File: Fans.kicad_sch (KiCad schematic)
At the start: 12 parts, among them Q1 NMOS, Q2 NMOS

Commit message: Initial layout with 1 pump, 2 temp, 1 flow all on front side
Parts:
- Q1, Q2: footprint Package_TO_SOT_SMD:LFPAK33 -> Package_TO_SOT_SMD:SOT-23
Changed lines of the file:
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@@
+	)
+	(symbol
+		(lib_id "power:GND")
+		(at 114.3 63.5 0)
+		(unit 1)
+		(exclude_from_sim no)
+		(in_bom yes)
+		(on_board yes)
+		(dnp no)
+		(fields_autoplaced yes)
+		(property "Reference" "#PWR016"
+			(at 114.3 69.85 0)
+			(effects
+				(font
+					(size 1.27 1.27)
+				)
+				(hide yes)
+			)
+		)
+		(property "Value" "GND"
+			(at 114.3 68.58 0)
+			(effects
+				(font
+					(size 1.27 1.27)
+				)
+			)
+		)
+		(property "Footprint" ""
+			(at 114.3 63.5 0)
+			(effects
+				(font
+					(size 1.27 1.27)
+				)
+				(hide yes)
+			)
+		)
+		(property "Datasheet" ""
+			(at 114.3 63.5 0)
+			(effects
+				(font
+					(size 1.27 1.27)
+				)
+				(hide yes)
+			)
+		)
+		(property "Description" "Power symbol creates a global label with name \"GND\" , ground"
+			(at 114.3 63.5 0)
+			(effects
+				(font
+					(size 1.27 1.27)
+				)
+				(hide yes)
+			)
+		)
+		(pin "1"
+		)
+		(instances
+			(project "PTN-PumpControlBoard"
+				(path "/591f46f8-eb1d-42dc-a4cb-8182eac4ef58/d90f7da4-ca39-48c6-8d97-b8d1e37c7dd0"
+					(reference "#PWR016")
+					(unit 1)
+				)
+			)
+		)
+	)
+	(symbol
+		(lib_id "Device:R_US")
+		(at 113.03 114.3 0)
+		(unit 1)
+		(exclude_from_sim no)
+		(in_bom yes)
+		(on_board yes)
+		(dnp no)
+		(property "Reference" "R8"
+			(at 115.57 113.0299 0)
+			(effects
+				(font
+					(size 1.27 1.27)
+				)
+				(justify left)
+			)
+		)
+		(property "Value" "1k"
+			(at 115.57 115.5699 0)
+			(effects
+				(font
+					(size 1.27 1.27)
+				)
+				(justify left)
+			)
+		)
+		(property "Footprint" "Resistor_SMD:R_0805_2012Metric"
+			(at 114.046 114.554 90)
+			(effects
+				(font
+					(size 1.27 1.27)
+				)
+				(hide yes)
+			)
+		)
+		(property "Datasheet" "~"
+			(at 113.03 114.3 0)
+			(effects
+				(font
+					(size 1.27 1.27)
+				)
+				(hide yes)
+			)
+		)
+		(property "Description" "Resistor, US symbol"
+			(at 113.03 114.3 0)
+			(effects
+				(font
+					(size 1.27 1.27)
+				)
+				(hide yes)
+			)
+		)
+		(pin "1"
+		)
+		(pin "2"
+		)
+		(instances
+			(project "PTN-PumpControlBoard"
+				(path "/591f46f8-eb1d-42dc-a4cb-8182eac4ef58/d90f7da4-ca39-48c6-8d97-b8d1e37c7dd0"
+					(reference "R8")
+					(unit 1)
+				)
+			)
+		)
+	)
+	(symbol
+		(lib_id "Device:D")
+		(at 52.07 38.1 270)
+		(unit 1)
+		(exclude_from_sim no)
+		(in_bom yes)
+		(on_board yes)
+		(dnp no)
+		(fields_autoplaced yes)
+		(property "Reference" "D1"
+			(at 54.61 36.8299 90)
+			(effects
+				(font
+					(size 1.27 1.27)
+				)
+				(justify left)
+			)
+		)
+		(property "Value" "1N4448W"
+			(at 54.61 39.3699 90)
+			(effects
+				(font
+					(size 1.27 1.27)
+				)
+				(justify left)
+			)
+		)
+		(property "Footprint" "Diode_SMD:D_SOD-323"
+			(at 52.07 38.1 0)
+			(effects
+				(font
+					(size 1.27 1.27)
+				)
+				(hide yes)
+			)
+		)
+		(property "Datasheet" "https://www.vishay.com/docs/85722/1n4448w.pdf"
+			(at 52.07 38.1 0)
+			(effects
+				(font
+					(size 1.27 1.27)
+				)
+				(hide yes)
+			)
+		)
+		(property "Description" "Diode"
+			(at 52.07 38.1 0)
+			(effects
+				(font
+					(size 1.27 1.27)
+				)
+				(hide yes)
+			)
+		)
+		(property "Sim.Device" "D"
+			(at 52.07 38.1 0)
+			(effects
+				(font
+					(size 1.27 1.27)
+				)
+				(hide yes)
+			)
+		)
+		(property "Sim.Pins" "1=K 2=A"
+			(at 52.07 38.1 0)
+			(effects
+				(font
+					(size 1.27 1.27)
+				)
+				(hide yes)
+			)
+		)
+		(pin "1"
+		)
+		(pin "2"
+		)
+		(instances
+			(project "PTN-PumpControlBoard"
+				(path "/591f46f8-eb1d-42dc-a4cb-8182eac4ef58/d90f7da4-ca39-48c6-8d97-b8d1e37c7dd0"
+					(reference "D1")
+					(unit 1)
+				)
+			)
+		)
 	)
 	(symbol
@@
 			)
 		)
-		(property "Footprint" "Package_TO_SOT_SMD:LFPAK33"
+		(property "Footprint" "Package_TO_SOT_SMD:SOT-23"
 			(at 66.04 50.8 0)
 			(effects
@@
 	)
 	(symbol
-		(lib_id "power:GND")
-		(at 114.3 63.5 0)
-		(unit 1)
-		(exclude_from_sim no)
-		(in_bom yes)
-		(on_board yes)
-		(dnp no)
-		(fields_autoplaced yes)
-		(property "Reference" "#PWR016"
-			(at 114.3 69.85 0)
-			(effects
-				(font
-					(size 1.27 1.27)
-				)
-				(hide yes)
-			)
-		)
-		(property "Value" "GND"
-			(at 114.3 68.58 0)
-			(effects
-				(font
-					(size 1.27 1.27)
-				)
-			)
-		)
-		(property "Footprint" ""
-			(at 114.3 63.5 0)
-			(effects
-				(font
-					(size 1.27 1.27)
-				)
-				(hide yes)
-			)
-		)
-		(property "Datasheet" ""
-			(at 114.3 63.5 0)
-			(effects
-				(font
-					(size 1.27 1.27)
-				)
-				(hide yes)
-			)
-		)
-		(property "Description" "Power symbol creates a global label with name \"GND\" , ground"
-			(at 114.3 63.5 0)
-			(effects
-				(font
-					(size 1.27 1.27)
-				)
-				(hide yes)
-			)
-		)
-		(pin "1"
-		)
-		(instances
-			(project "PTN-PumpControlBoard"
-				(path "/591f46f8-eb1d-42dc-a4cb-8182eac4ef58/d90f7da4-ca39-48c6-8d97-b8d1e37c7dd0"
-					(reference "#PWR016")
-					(unit 1)
-				)
-			)
-		)
-	)
-	(symbol
-		(lib_id "Device:R_US")
-		(at 113.03 114.3 0)
-		(unit 1)
-		(exclude_from_sim no)
-		(in_bom yes)
-		(on_board yes)
-		(dnp no)
-		(property "Reference" "R8"
-			(at 115.57 113.0299 0)
-			(effects
-				(font
-					(size 1.27 1.27)
-				)
-				(justify left)
-			)
-		)
-		(property "Value" "1k"
-			(at 115.57 115.5699 0)
-			(effects
-				(font
-					(size 1.27 1.27)
-				)
-				(justify left)
-			)
-		)
-		(property "Footprint" "Resistor_SMD:R_0805_2012Metric"
-			(at 114.046 114.554 90)
-			(effects
-				(font
-					(size 1.27 1.27)
-				)
-				(hide yes)
-			)
-		)
-		(property "Datasheet" "~"
-			(at 113.03 114.3 0)
-			(effects
-				(font
-					(size 1.27 1.27)
-				)
-				(hide yes)
-			)
-		)
-		(property "Description" "Resistor, US symbol"
-			(at 113.03 114.3 0)
-			(effects
-				(font
-					(size 1.27 1.27)
-				)
-				(hide yes)
-			)
-		)
-		(pin "1"
-		)
-		(pin "2"
-		)
-		(instances
-			(project "PTN-PumpControlBoard"
-				(path "/591f46f8-eb1d-42dc-a4cb-8182eac4ef58/d90f7da4-ca39-48c6-8d97-b8d1e37c7dd0"
-					(reference "R8")
-					(unit 1)
-				)
-			)
-		)
-	)
-	(symbol
-		(lib_id "Device:D")
-		(at 52.07 38.1 270)
-		(unit 1)
-		(exclude_from_sim no)
-		(in_bom yes)
-		(on_board yes)
-		(dnp no)
-		(fields_autoplaced yes)
-		(property "Reference" "D1"
-			(at 54.61 36.8299 90)
-			(effects
-				(font
-					(size 1.27 1.27)
-				)
-				(justify left)
-			)
-		)
-		(property "Value" "1N4448W"
-			(at 54.61 39.3699 90)
-			(effects
-				(font
-					(size 1.27 1.27)
-				)
-				(justify left)
-			)
-		)
-		(property "Footprint" "Diode_SMD:D_SOD-323"
-			(at 52.07 38.1 0)
-			(effects
-				(font
-					(size 1.27 1.27)
-				)
-				(hide yes)
-			)
-		)
-		(property "Datasheet" "https://www.vishay.com/docs/85722/1n4448w.pdf"
-			(at 52.07 38.1 0)
-			(effects
-				(font
-					(size 1.27 1.27)
-				)
-				(hide yes)
-			)
-		)
-		(property "Description" "Diode"
-			(at 52.07 38.1 0)
-			(effects
-				(font
-					(size 1.27 1.27)
-				)
-				(hide yes)
-			)
-		)
-		(property "Sim.Device" "D"
-			(at 52.07 38.1 0)
-			(effects
-				(font
-					(size 1.27 1.27)
-				)
-				(hide yes)
-			)
-		)
-		(property "Sim.Pins" "1=K 2=A"
-			(at 52.07 38.1 0)
-			(effects
-				(font
-					(size 1.27 1.27)
-				)
-				(hide yes)
-			)
-		)
-		(pin "1"
-		)
-		(pin "2"
-		)
-		(instances
-			(project "PTN-PumpControlBoard"
-				(path "/591f46f8-eb1d-42dc-a4cb-8182eac4ef58/d90f7da4-ca39-48c6-8d97-b8d1e37c7dd0"
-					(reference "D1")
-					(unit 1)
-				)
-			)
-		)
-	)
-	(symbol
 		(lib_id "Connector_Generic:Conn_01x03")
 		(at 78.74 38.1 0)
@@
 			)
 		)
-		(property "Footprint" "Package_TO_SOT_SMD:LFPAK33"
+		(property "Footprint" "Package_TO_SOT_SMD:SOT-23"
 			(at 64.77 120.65 0)
 			(effects

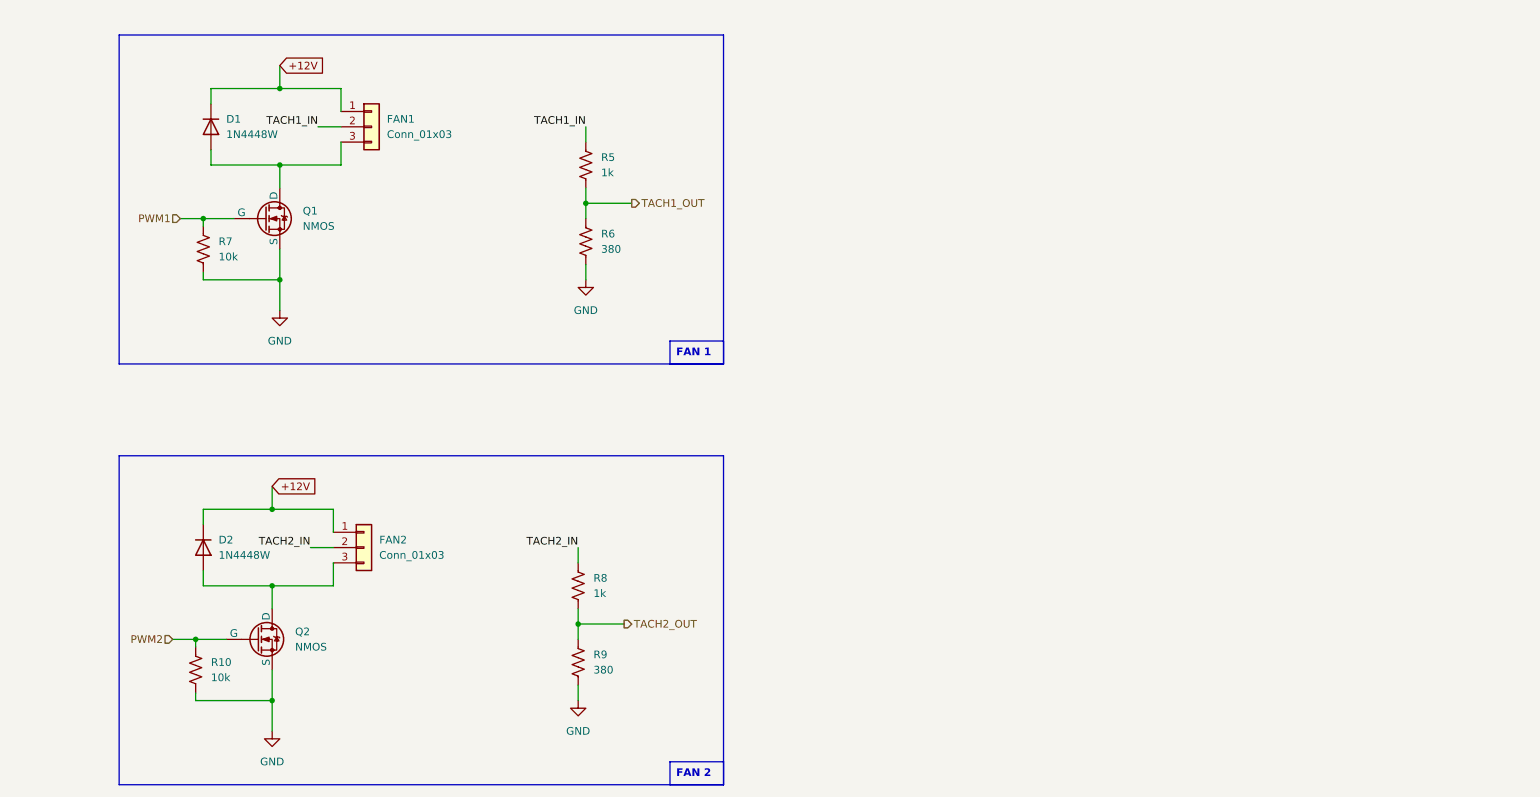
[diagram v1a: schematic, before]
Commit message: schematic with 12V components, unigain buffers & extra temp sensor
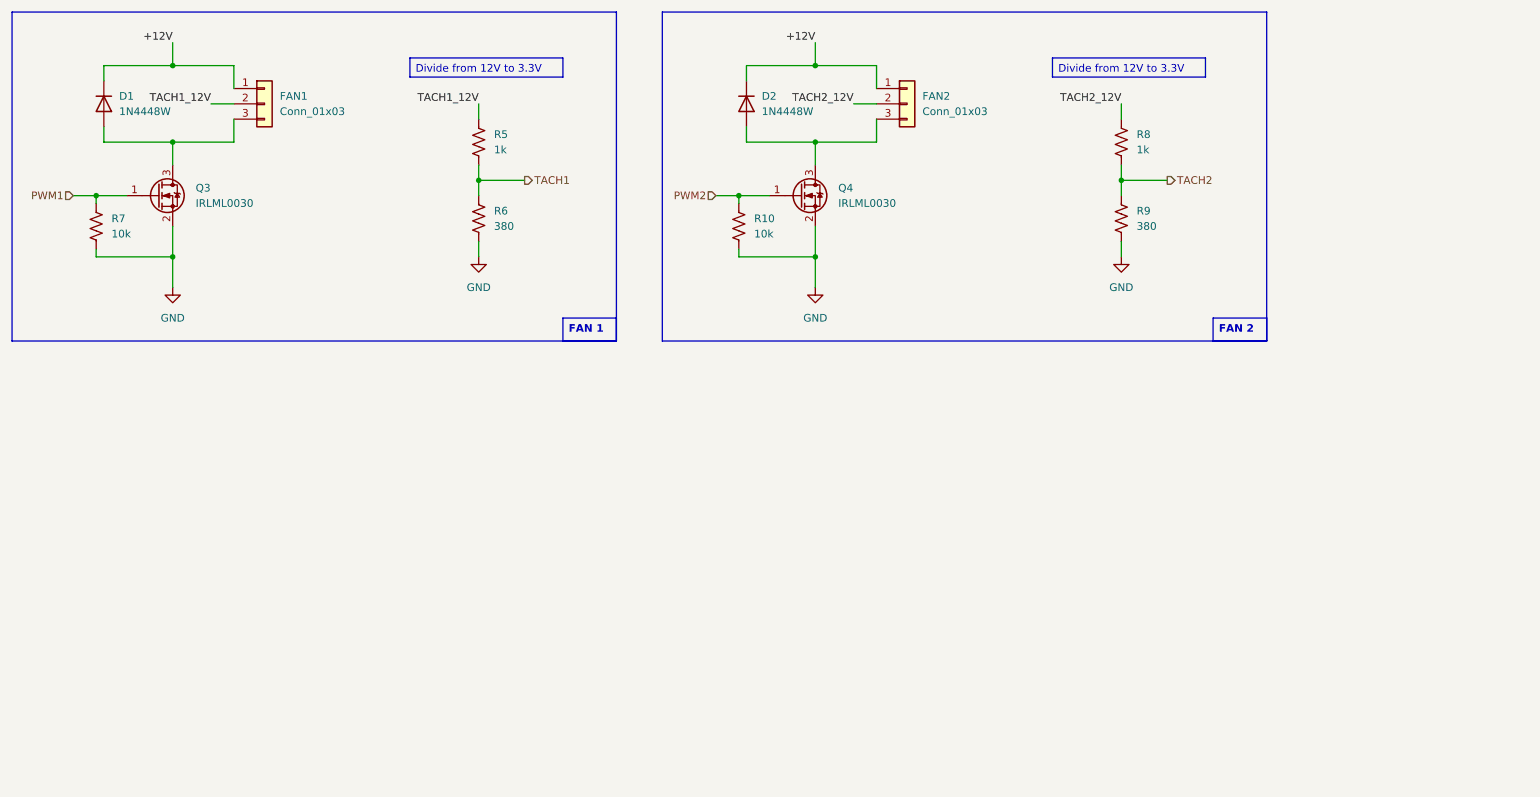
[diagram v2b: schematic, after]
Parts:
- removed Q1, Q2: NMOS, Package_TO_SOT_SMD:SOT-23, symbol Simulation_SPICE:NMOS
- added Q3, Q4: IRLML0030, Package_TO_SOT_SMD:SOT-23, symbol Transistor_FET:IRLML0030
- FAN1, FAN2: footprint UTSVT_Connectors:Molex_MicroFit3.0_1x3xP3.00mm_PolarizingPeg_Vertical -> Connector_Molex:Molex_Nano-Fit_105309-xx03_1x03_P2.50mm_Vertical
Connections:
- net GND: now also Q3.2 (S), Q4.2 (S)
- net PWM1: now also Q3.1 (G)
- net PWM2: now also Q4.1 (G)
- net at D1.2 (A), FAN1.3 (Pin_3): now also Q3.3 (D)
- net at D2.2 (A), FAN2.3 (Pin_3): now also Q4.3 (D)
- net TACH1_IN renamed TACH1_12V
- net TACH1_OUT renamed TACH1
- net TACH2_IN renamed TACH2_12V
- net TACH2_OUT renamed TACH2
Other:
- moved on the sheet: D1, D2, FAN1, FAN2, R10, R5, R6, R7, R8, R9

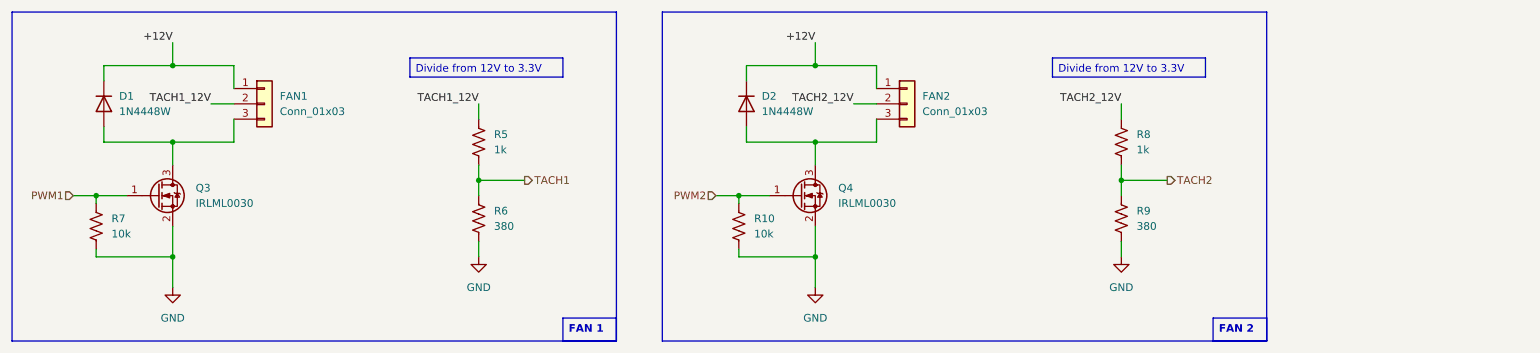
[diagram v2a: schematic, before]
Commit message: repicked parts to be 24V tolerant and changed corresponding circuitry
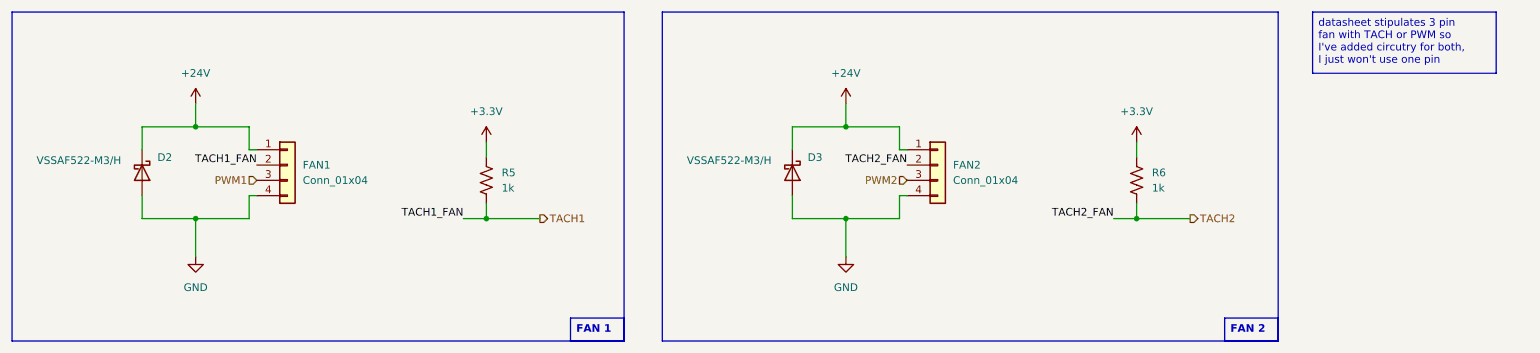
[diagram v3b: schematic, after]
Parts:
- removed D1, D2: 1N4448W, Diode_SMD:D_SOD-323, symbol Device:D
- removed FAN1, FAN2: Conn_01x03, Connector_Molex:Molex_Nano-Fit_105309-xx03_1x03_P2.50mm_Vertical, symbol Connector_Generic:Conn_01x03
- removed Q3, Q4: IRLML0030, Package_TO_SOT_SMD:SOT-23, symbol Transistor_FET:IRLML0030
- removed R10, R7: 10k, Resistor_SMD:R_0805_2012Metric, symbol Device:R_US
- removed R8: 1k, Resistor_SMD:R_0805_2012Metric, symbol Device:R_US
- removed R9: 380, Resistor_SMD:R_0805_2012Metric, symbol Device:R_US
- added D2, D3: VSSAF522-M3/H, UTSVT_Passive:DO-221AC, symbol Diode:C3D25170H
- added FAN1, FAN2: Conn_01x04, Connector_Molex:Molex_Nano-Fit_105309-xx04_1x04_P2.50mm_Vertical, symbol Connector_Generic:Conn_01x04
- R6: value 380 -> 1k
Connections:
- net GND: now also D2.2 (A), D3.2 (A), FAN1.4 (Pin_4), FAN2.4 (Pin_4); no longer R6.2
- net PWM1: now also FAN1.3 (Pin_3)
- net PWM2: now also FAN2.3 (Pin_3)
- net TACH1: now also FAN1.2 (Pin_2); no longer R6.1
- net TACH2: now also R6.2, FAN2.2 (Pin_2)
- net TACH1_12V renamed +3.3V
- net +3.3V: now also R6.1
- new net +24V: D2.1 (K), D3.1 (K), FAN1.1 (Pin_1), FAN2.1 (Pin_1)
